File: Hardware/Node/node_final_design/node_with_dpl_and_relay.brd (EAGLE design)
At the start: 101.3 x 85.1 mm, 57 parts, among them K1 G6RS, T1 FDN340P, U1 NCP1117ST50T3G, U2 LP2985-33DBVR, U5 LMV358IDGKR, X1 POWERSUPPLY_DC21MMX, Y1 8Mhz, Y2 CSTCE16M0V53-R0 16MHZ

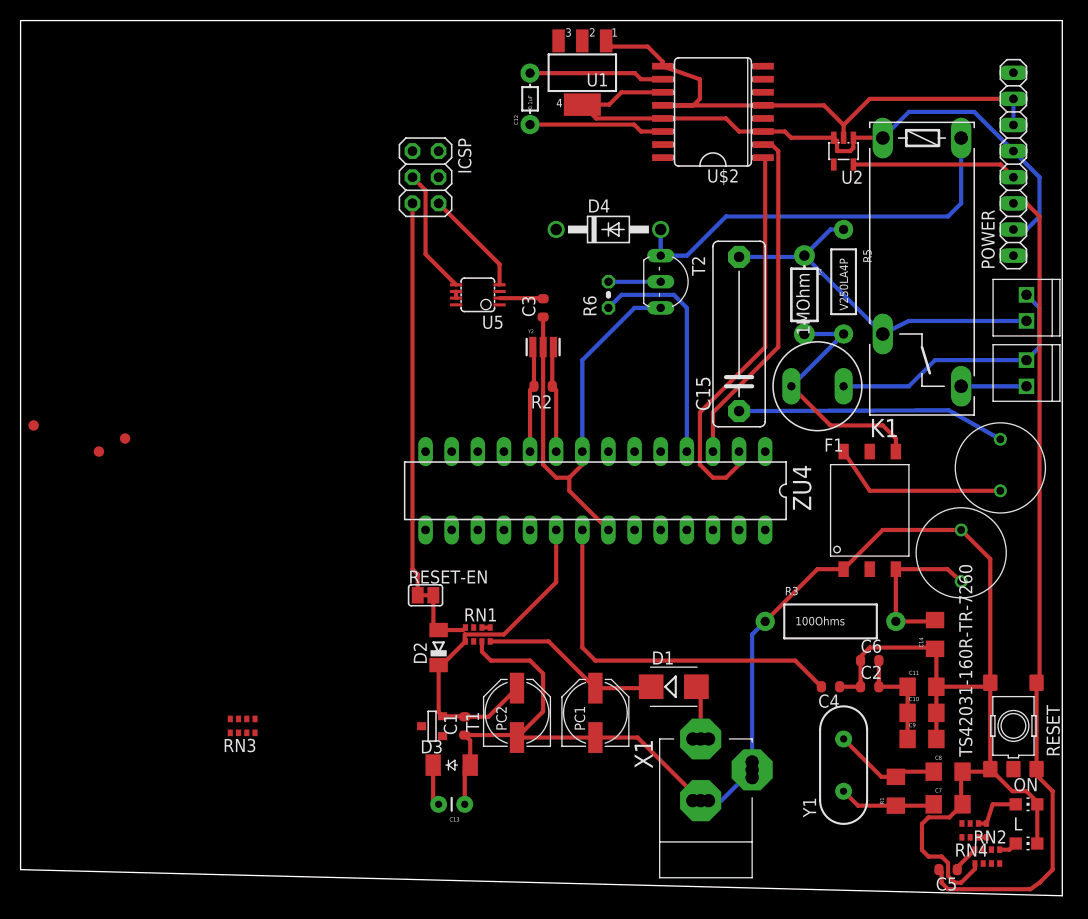
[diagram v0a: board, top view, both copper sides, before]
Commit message: node pcb done
should work
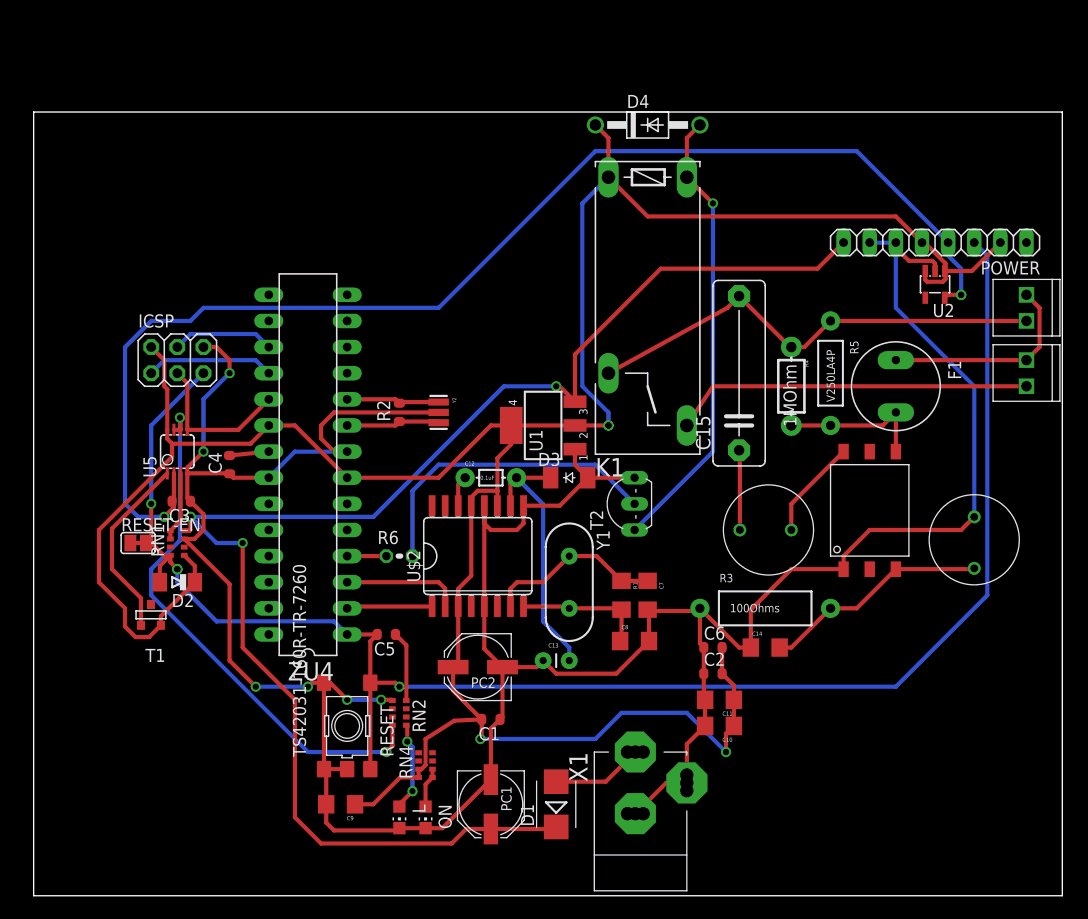
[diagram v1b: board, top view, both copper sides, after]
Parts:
- removed FD1, FD2, FD3: FIDUCIALMOUNT, SmartPrj:FIDUCIA-MOUNT
- removed RN3: 22R, resistor-dil:CAY16
- moved RESET 64.8 mm to (31.8, 14.0)
- moved C4 62.3 mm to (20.3, 39.4), turned to 90 degrees
- moved L 61.0 mm to (36.8, 5.08), turned to 180 degrees
- moved C5 59.2 mm to (35.6, 22.9)
- moved RN2 58.8 mm to (36.8, 15.2), turned to 90 degrees
- moved ON 58.4 mm to (39.4, 5.08), turned to 180 degrees
- moved C9 56.9 mm to (31.1, 6.35), turned to 180 degrees
- moved RN4 53.7 mm to (39.4, 10.2), turned to 270 degrees
- moved U$2 48.9 mm to (44.5, 30.5), turned to 0 degrees
- moved C3 39.9 mm to (15.6, 35.8), turned to 180 degrees
- moved C12 37.0 mm to (45.7, 38.1), turned to 0 degrees
- moved C7 35.6 mm to (61.0, 26.7), turned to 270 degrees
- moved U1 34.5 mm to (50.8, 43.2), turned to 90 degrees
- moved C8 33.0 mm to (59.7, 22.2)
- moved U5 32.9 mm to (15.2, 40.6), turned to 0 degrees
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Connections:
- removed net 5-GND: RESET.5
- net GND: now also RESET.5
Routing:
- net +5V: track 112.2 -> 263.0 mm, vias 0 -> 3
- net VIN: track 17.6 -> 142.4 mm, vias 0 -> 3
- net +3V3: track 20.3 -> 125.9 mm, vias 0 -> 2
- net L13: track 0.65 -> 52.3 mm, vias 0 -> 2
- net RESET: track 126.6 -> 162.5 mm, vias 0 -> 3
- net AREF: track 36.2 -> 3.83 mm
- net N$14: track 38.7 -> 8.33 mm
- net N$11: track 6.35 -> 35.1 mm
- net N$16: track 5.08 -> 30.6 mm
- net N$13: track 33.6 -> 11.5 mm
- net N$15: track 22.6 -> 3.81 mm
- net N$9: track 26.1 -> 7.78 mm
- net GATE_CMD: track 0.00 -> 18.2 mm
- net MISO: track 0.00 -> 12.5 mm
- net N$5: track 13.2 -> 3.00 mm
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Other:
- board size 101.3 x 85.1 mm -> 100 x 76.2 mm
